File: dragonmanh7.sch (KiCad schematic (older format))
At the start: 103 parts, among them J1 10118194-0001LF, J10 Conn_02x12_Odd_Even, J11 Conn_02x02_Odd_Even, J12 VBAT+, J13 PROTO1, J14 VBATG, J18 PROTO1, J2 10118194-0001LF, J3 RJ45_Amphenol_RJMG1BD3B8K1ANR, J4 Micro_SD_Card, J5 Screw_Terminal_01x06, J6 Conn_02x12_Odd_Even, J7 10118194-0001LF, J8 Screw_Terminal_01x02, J9 Conn_02x12_Odd_Even, SW1 RESET, SW2 PC13, U1 STM32H743VITx, U10 USBLC6-2SC6, U11 SN6505, U12 TCAN332, U13 ISL83483, U2 KSZ8081RNA, U3 ISO1050DUB, U4 ISO3082DW, U5 S25FL127SABMFI101, U6 AP63203, U7 USBLC6-2SC6, U8 STM32F042F6Px, U9 USBLC6-2SC6, Y1 8MHz, Y2 32.768KHz, Y3 25MHz

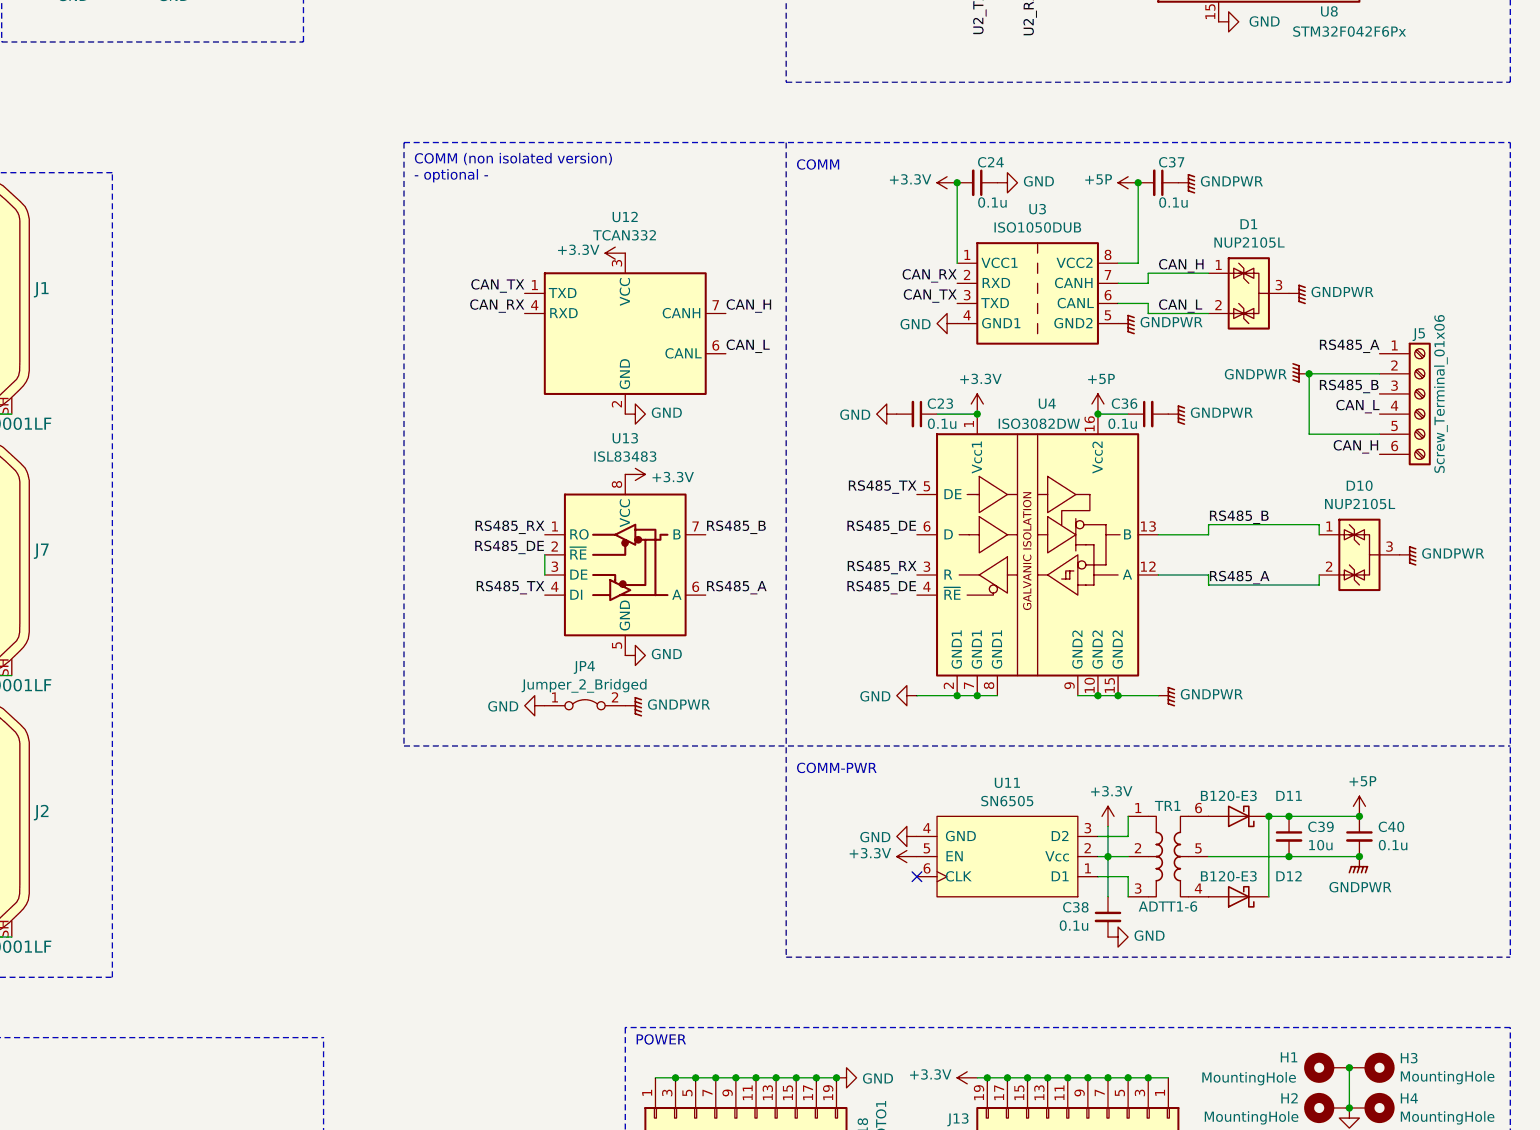
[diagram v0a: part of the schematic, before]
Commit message: Update images and README
Signed-off-by: Martin Ribelotta <martinribelotta@gmail.com>
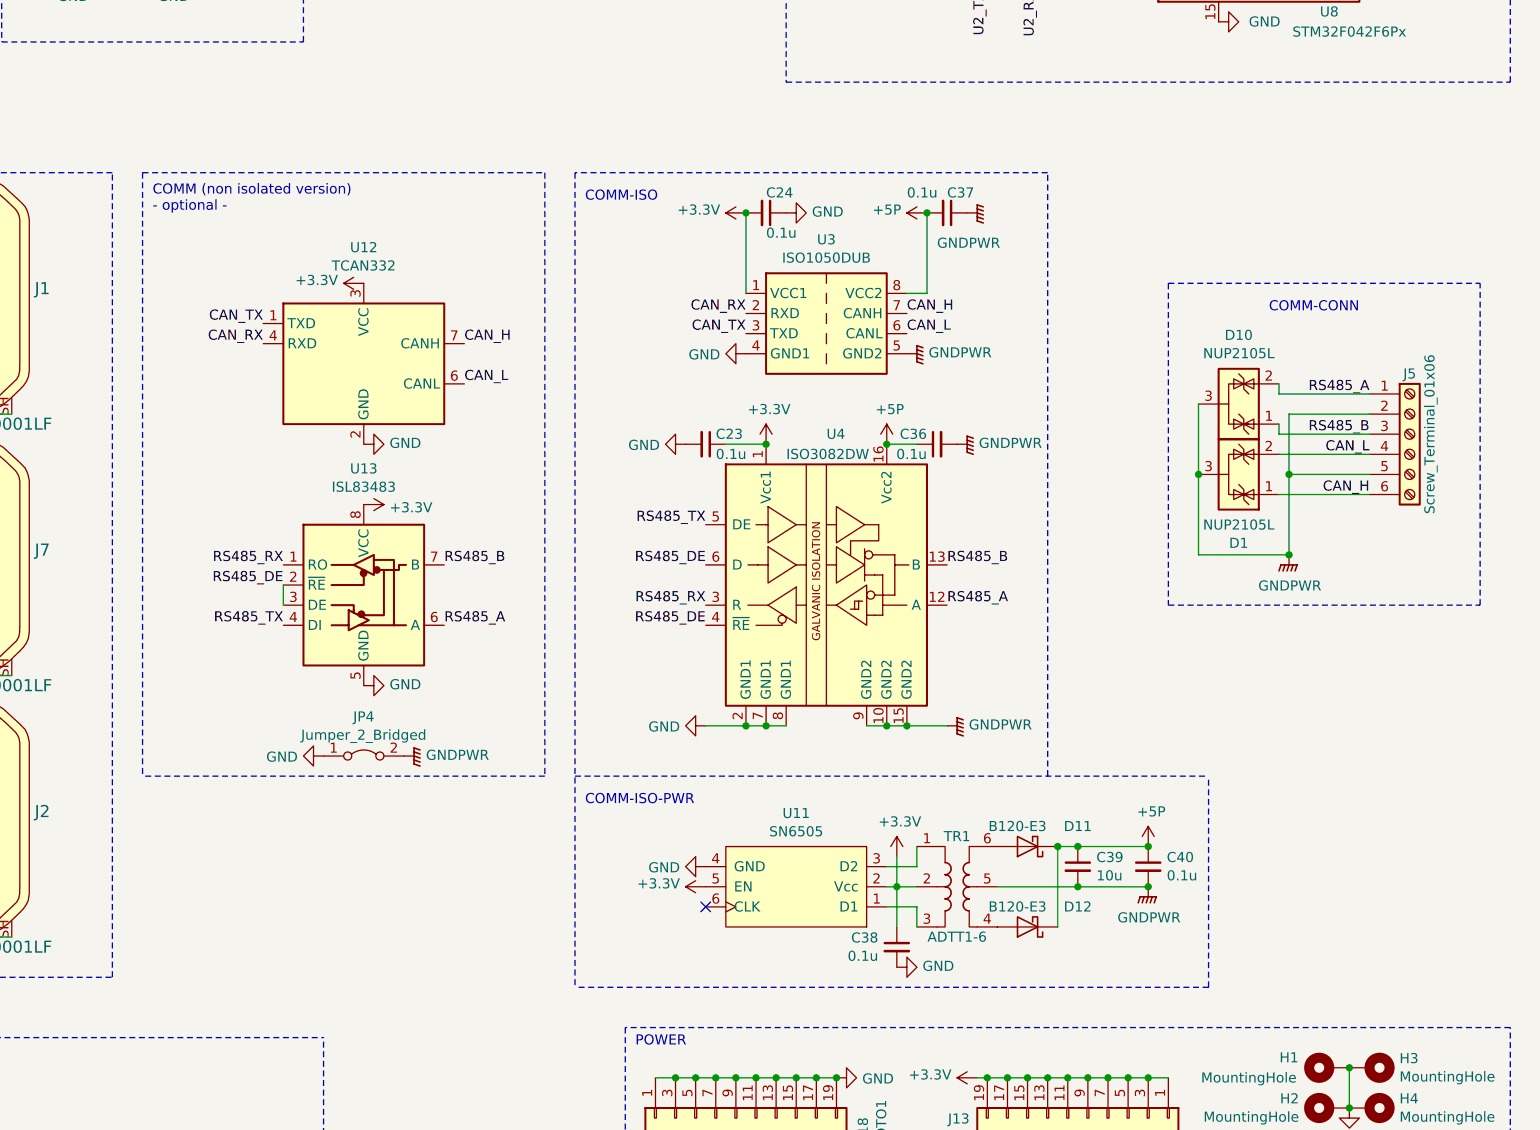
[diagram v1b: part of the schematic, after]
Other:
- note added: "COMM-CONN"
- note added: "COMM-ISO"
- note added: "COMM-ISO-PWR"
- note removed: "COMM"
- note removed: "COMM-PWR"
- moved on the sheet: C23, C24, C36, C37, C38, C39, C40, D1, D10, D11, D12, J5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
